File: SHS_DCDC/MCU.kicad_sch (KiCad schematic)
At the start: 15 parts, among them J3 Conn_ARM_JTAG_SWD_10, J4 Conn_01x02_Male, U6 ESP32-S2-MINI-1, U8 MIC5501-3.0YM5, Y1 2-SMD no lead

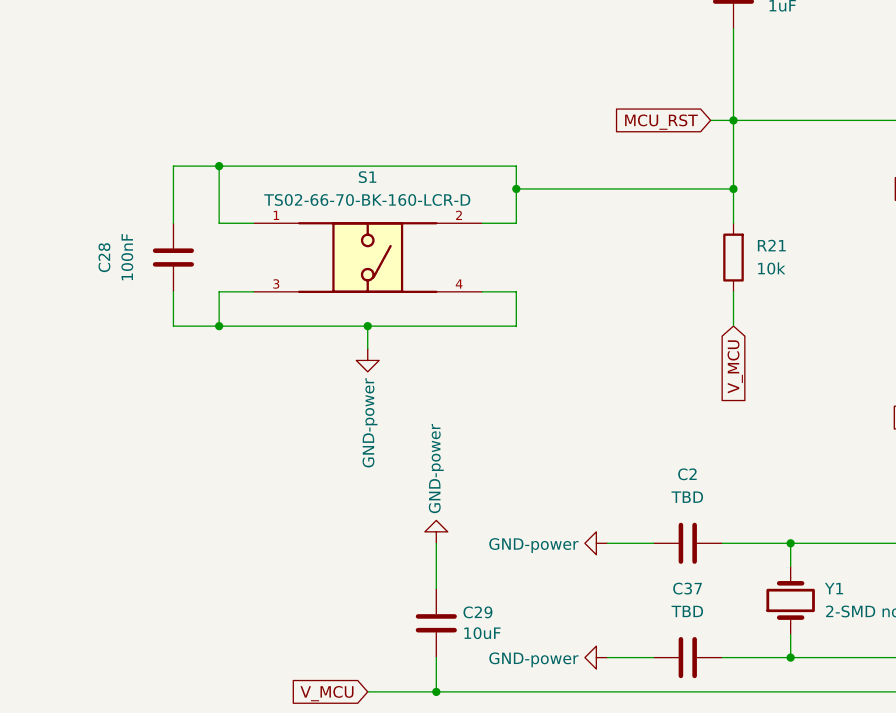
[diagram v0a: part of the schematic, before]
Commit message: 3D rendering progress
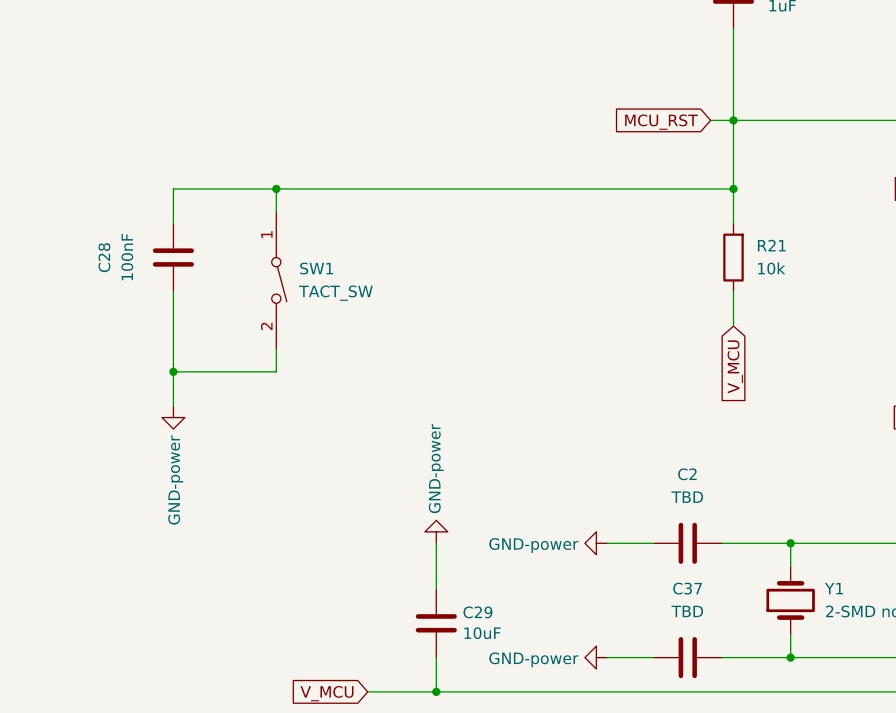
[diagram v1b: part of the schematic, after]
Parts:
- removed S1: TS02-66-70-BK-160-LCR-D, SW_TS02-66-70-BK-160-LCR-D, symbol SHS_DCDC:TS02-66-70-BK-160-LCR-D
- added SW1: TACT_SW, SHS_DCDC:ESWITCH_TL1105, symbol SHS_DCDC:TACT_SW
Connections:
- net GND: now also SW1.2
- net MCU_RST: now also SW1.1
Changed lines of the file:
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@@
 (kicad_sch (version 20211123) (generator eeschema)
   (paper "A4")
-  (junction (at 41.91 102.87) (diameter 0) (color 0 0 0 0)
-  )
   (junction (at 259.08 80.01) (diameter 0) (color 0 0 0 0)
   )
@@
   (junction (at 66.04 143.51) (diameter 0) (color 0 0 0 0)
   )
-  (junction (at 58.42 102.87) (diameter 0) (color 0 0 0 0)
+  (junction (at 36.83 107.95) (diameter 0) (color 0 0 0 0)
+  )
+  (junction (at 48.26 87.63) (diameter 0) (color 0 0 0 0)
   )
   (junction (at 165.1 31.75) (diameter 0) (color 0 0 0 0)
@@
   (junction (at 105.41 127) (diameter 0) (color 0 0 0 0)
   )
-  (junction (at 74.93 87.63) (diameter 0) (color 0 0 0 0)
-  )
-  (junction (at 41.91 85.09) (diameter 0) (color 0 0 0 0)
-  )
   (junction (at 105.41 139.7) (diameter 0) (color 0 0 0 0)
   )
@@
     (stroke (width 0) (type default) (color 0 0 0 0))
   )
-  (wire (pts (xy 36.83 102.87) (xy 41.91 102.87))
-    (stroke (width 0) (type default) (color 0 0 0 0))
-  )
   (wire (pts (xy 259.08 80.01) (xy 259.08 66.04))
     (stroke (width 0) (type default) (color 0 0 0 0))
@@
     (stroke (width 0) (type default) (color 0 0 0 0))
   )
-  (wire (pts (xy 41.91 85.09) (xy 74.93 85.09))
-    (stroke (width 0) (type default) (color 0 0 0 0))
-  )
-  (wire (pts (xy 36.83 91.44) (xy 36.83 85.09))
+  (wire (pts (xy 36.83 91.44) (xy 36.83 87.63))
     (stroke (width 0) (type default) (color 0 0 0 0))
   )
@@
     (stroke (width 0) (type default) (color 0 0 0 0))
   )
+  (wire (pts (xy 36.83 107.95) (xy 36.83 111.76))
+    (stroke (width 0) (type default) (color 0 0 0 0))
+  )
   (wire (pts (xy 118.11 130.81) (xy 118.11 127))
     (stroke (width 0) (type default) (color 0 0 0 0))
   )
-  (wire (pts (xy 74.93 91.44) (xy 71.12 91.44))
-    (stroke (width 0) (type default) (color 0 0 0 0))
-  )
   (wire (pts (xy 118.11 127) (xy 105.41 127))
     (stroke (width 0) (type default) (color 0 0 0 0))
@@
     (stroke (width 0) (type default) (color 0 0 0 0))
   )
-  (wire (pts (xy 45.72 91.44) (xy 41.91 91.44))
-    (stroke (width 0) (type default) (color 0 0 0 0))
-  )
   (wire (pts (xy 215.9 80.01) (xy 259.08 80.01))
     (stroke (width 0) (type default) (color 0 0 0 0))
   )
+  (wire (pts (xy 48.26 87.63) (xy 99.06 87.63))
+    (stroke (width 0) (type default) (color 0 0 0 0))
+  )
   (wire (pts (xy 92.71 160.02) (xy 143.51 160.02))
     (stroke (width 0) (type default) (color 0 0 0 0))
@@
     (stroke (width 0) (type default) (color 0 0 0 0))
   )
-  (wire (pts (xy 74.93 99.06) (xy 74.93 102.87))
-    (stroke (width 0) (type default) (color 0 0 0 0))
-  )
   (wire (pts (xy 118.11 137.16) (xy 143.51 137.16))
     (stroke (width 0) (type default) (color 0 0 0 0))
@@
     (stroke (width 0) (type default) (color 0 0 0 0))
   )
-  (wire (pts (xy 41.91 102.87) (xy 41.91 99.06))
-    (stroke (width 0) (type default) (color 0 0 0 0))
-  )
   (wire (pts (xy 215.9 120.65) (xy 227.33 120.65))
     (stroke (width 0) (type default) (color 0 0 0 0))
@@
     (stroke (width 0) (type default) (color 0 0 0 0))
   )
-  (wire (pts (xy 36.83 85.09) (xy 41.91 85.09))
+  (wire (pts (xy 48.26 87.63) (xy 48.26 90.17))
+    (stroke (width 0) (type default) (color 0 0 0 0))
+  )
+  (wire (pts (xy 36.83 87.63) (xy 48.26 87.63))
     (stroke (width 0) (type default) (color 0 0 0 0))
   )
@@
     (stroke (width 0) (type default) (color 0 0 0 0))
   )
-  (wire (pts (xy 36.83 99.06) (xy 36.83 102.87))
-    (stroke (width 0) (type default) (color 0 0 0 0))
-  )
   (wire (pts (xy 143.51 149.86) (xy 92.71 149.86))
     (stroke (width 0) (type default) (color 0 0 0 0))
@@
     (stroke (width 0) (type default) (color 0 0 0 0))
   )
-  (wire (pts (xy 71.12 99.06) (xy 74.93 99.06))
-    (stroke (width 0) (type default) (color 0 0 0 0))
-  )
   (wire (pts (xy 246.38 25.4) (xy 246.38 22.86))
     (stroke (width 0) (type default) (color 0 0 0 0))
@@
     (stroke (width 0) (type default) (color 0 0 0 0))
   )
+  (wire (pts (xy 48.26 107.95) (xy 36.83 107.95))
+    (stroke (width 0) (type default) (color 0 0 0 0))
+  )
   (wire (pts (xy 215.9 135.89) (xy 227.33 135.89))
     (stroke (width 0) (type default) (color 0 0 0 0))
@@
     (stroke (width 0) (type default) (color 0 0 0 0))
   )
-  (wire (pts (xy 74.93 87.63) (xy 74.93 91.44))
-    (stroke (width 0) (type default) (color 0 0 0 0))
-  )
   (wire (pts (xy 215.9 82.55) (xy 245.11 82.55))
     (stroke (width 0) (type default) (color 0 0 0 0))
@@
     (stroke (width 0) (type default) (color 0 0 0 0))
   )
-  (wire (pts (xy 58.42 105.41) (xy 58.42 102.87))
+  (wire (pts (xy 36.83 99.06) (xy 36.83 107.95))
     (stroke (width 0) (type default) (color 0 0 0 0))
   )
@@
     (stroke (width 0) (type default) (color 0 0 0 0))
   )
-  (wire (pts (xy 74.93 85.09) (xy 74.93 87.63))
-    (stroke (width 0) (type default) (color 0 0 0 0))
-  )
-  (wire (pts (xy 58.42 102.87) (xy 74.93 102.87))
-    (stroke (width 0) (type default) (color 0 0 0 0))
-  )
-  (wire (pts (xy 41.91 99.06) (xy 45.72 99.06))
+  (wire (pts (xy 48.26 105.41) (xy 48.26 107.95))
     (stroke (width 0) (type default) (color 0 0 0 0))
   )
@@
     (stroke (width 0) (type default) (color 0 0 0 0))
   )
-  (wire (pts (xy 41.91 91.44) (xy 41.91 85.09))
-    (stroke (width 0) (type default) (color 0 0 0 0))
-  )
   (wire (pts (xy 246.38 55.88) (xy 246.38 62.23))
     (stroke (width 0) (type default) (color 0 0 0 0))
@@
   )
   (wire (pts (xy 66.04 143.51) (xy 58.42 143.51))
-    (stroke (width 0) (type default) (color 0 0 0 0))
-  )
-  (wire (pts (xy 74.93 87.63) (xy 99.06 87.63))
-    (stroke (width 0) (type default) (color 0 0 0 0))
-  )
-  (wire (pts (xy 41.91 102.87) (xy 58.42 102.87))
     (stroke (width 0) (type default) (color 0 0 0 0))
   )
@@
     (pin "9")
   )
-  (symbol (lib_id "SHS_DCDC:GND-power") (at 58.42 105.41 0) (unit 1)
-    (in_bom yes) (on_board yes)
-    (property "Reference" "#PWR0119" (id 0) (at 58.42 111.76 0)
-      (effects (font (size 1.27 1.27)) hide)
-    )
-    (property "Value" "GND-power" (id 1) (at 58.547 108.6612 90)
-      (effects (font (size 1.27 1.27)) (justify right))
-    )
-    (property "Footprint" "" (id 2) (at 58.42 105.41 0)
-      (effects (font (size 1.27 1.27)) hide)
-    )
-    (property "Datasheet" "" (id 3) (at 58.42 105.41 0)
+  (symbol (lib_id "SHS_DCDC:GND-power") (at 36.83 111.76 0) (unit 1)
+    (in_bom yes) (on_board yes)
+    (property "Reference" "#PWR0119" (id 0) (at 36.83 118.11 0)
+      (effects (font (size 1.27 1.27)) hide)
+    )
+    (property "Value" "GND-power" (id 1) (at 36.957 115.0112 90)
+      (effects (font (size 1.27 1.27)) (justify right))
+    )
+    (property "Footprint" "" (id 2) (at 36.83 111.76 0)
+      (effects (font (size 1.27 1.27)) hide)
+    )
+    (property "Datasheet" "" (id 3) (at 36.83 111.76 0)
       (effects (font (size 1.27 1.27)) hide)
     )
@@
     (pin "2")
   )
-  (symbol (lib_id "SHS_DCDC:TS02-66-70-BK-160-LCR-D") (at 58.42 95.25 0) (unit 1)
-    (in_bom yes) (on_board yes) (fields_autoplaced)
-    (property "Reference" "S1" (id 0) (at 58.42 86.36 0))
-    (property "Value" "TS02-66-70-BK-160-LCR-D" (id 1) (at 58.42 88.9 0))
-    (property "Footprint" "SW_TS02-66-70-BK-160-LCR-D" (id 2) (at 58.42 87.63 0)
-      (effects (font (size 1.27 1.27)) (justify bottom) hide)
-    )
-    (property "Datasheet" "" (id 3) (at 58.42 95.25 0)
-      (effects (font (size 1.27 1.27)) hide)
-    )
-    (property "MANUFACTURER" "CUI Devices" (id 4) (at 46.99 90.17 0)
-      (effects (font (size 1.27 1.27)) (justify bottom) hide)
-    )
-    (property "PARTREV" "1.0" (id 5) (at 58.42 95.25 0)
-      (effects (font (size 1.27 1.27)) (justify bottom) hide)
-    )
-    (property "STANDARD" "Manufacturer Recommendations" (id 6) (at 57.15 85.09 0)
-      (effects (font (size 1.27 1.27)) (justify bottom) hide)
-    )
-    (pin "1")
-    (pin "2")
-    (pin "3")
-    (pin "4")
-  )
   (symbol (lib_id "SHS_DCDC:GND-power") (at 179.07 53.34 0) (unit 1)
     (in_bom yes) (on_board yes)
@@
       (effects (font (size 1.27 1.27)) hide)
     )
+    (pin "1")
+    (pin "2")
+  )
+  (symbol (lib_id "SHS_DCDC:TACT_SW") (at 48.26 97.79 270) (unit 1)
+    (in_bom yes) (on_board yes) (fields_autoplaced)
+    (property "Reference" "SW1" (id 0) (at 50.8 96.5199 90)
+      (effects (font (size 1.27 1.27)) (justify left))
+    )
+    (property "Value" "TACT_SW" (id 1) (at 50.8 99.0599 90)
+      (effects (font (size 1.27 1.27)) (justify left))
+    )
+    (property "Footprint" "SHS_DCDC:ESWITCH_TL1105" (id 2) (at 48.26 97.79 0)
+      (effects (font (size 1.27 1.27)) hide)
+    )
+    (property "Datasheet" "~" (id 3) (at 48.26 97.79 0)
+      (effects (font (size 1.27 1.27)) hide)
+    )
